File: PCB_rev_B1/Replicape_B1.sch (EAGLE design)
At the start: 233 parts, among them IC1 TMC2100-LA, IC10 74AHC1G126DCK, IC11 74AHC1G126DCK, IC12 TMC2100-LA, IC13 74AHC1G126DCK, IC14 74AHC1G126DCK, IC15 TMC2100-LA, IC16 74AHC1G126DCK, IC17 74AHC1G126DCK, IC2 TMC2100-LA, IC3 74AHC1G126DCK, IC4 74AHC1G126DCK, IC5 TMC2100-LA, IC6 74AHC1G126DCK, IC7 74AHC1G126DCK, IC8 74AHC1G126DCK, IC9 74AHC1G126DCK, P8 F-2X23-, P9 F-2X23-, Q1 AON6758, Q2 AON6758, Q3 AON6758, U1 SN74AHC595PW, U10 RT8268, U11 PCA9685PW, U18 CAT24C256, U19 CD4050BD, U2 SN74AHC595PW, U3 SN74AHC595PW, U4 SN74AHC595PW, U5 SN74AHC595PW, U6 MCP16321, X1 22-05-7038-03, X10 22-05-7038-03, X11 22-05-7028-02, X12 22-05-7048-04, X13 22-05-7038-03, X14 22-05-7048-04, X15 22-05-7048-04, X16 22-05-7048-04, X17 22-05-7048-04, X18 22-05-7048-04, X19 22-05-7038-03, X2 MSTBA4, X20 MSTBA4, X21 MSTBA2, X22 22-05-7038-03, X23 22-05-7038-03, X3 MSTBA2, X4 22-05-7028-02, X5 22-05-7028-02, X6 22-05-7028-02, X7 22-05-7028-02, X8 22-05-7028-02, X9 22-05-7028-02

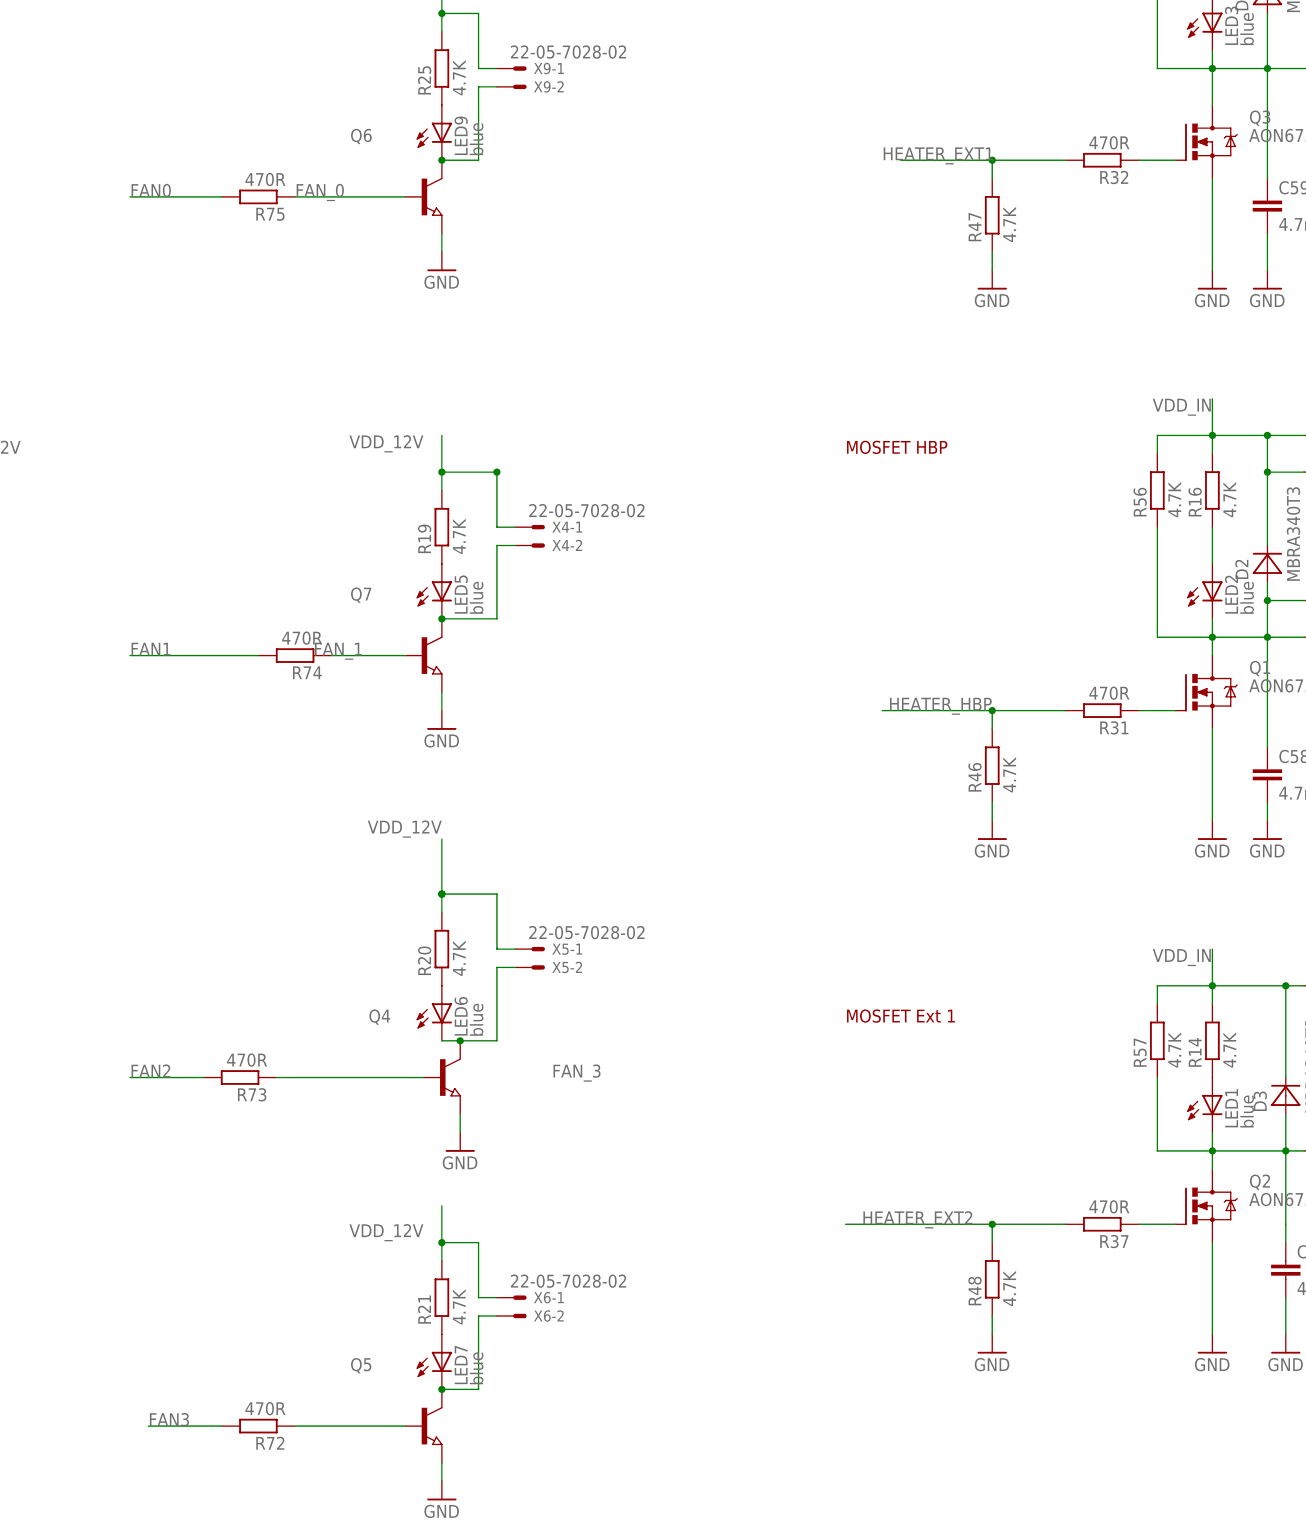
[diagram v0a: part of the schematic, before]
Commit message: Added eagleup
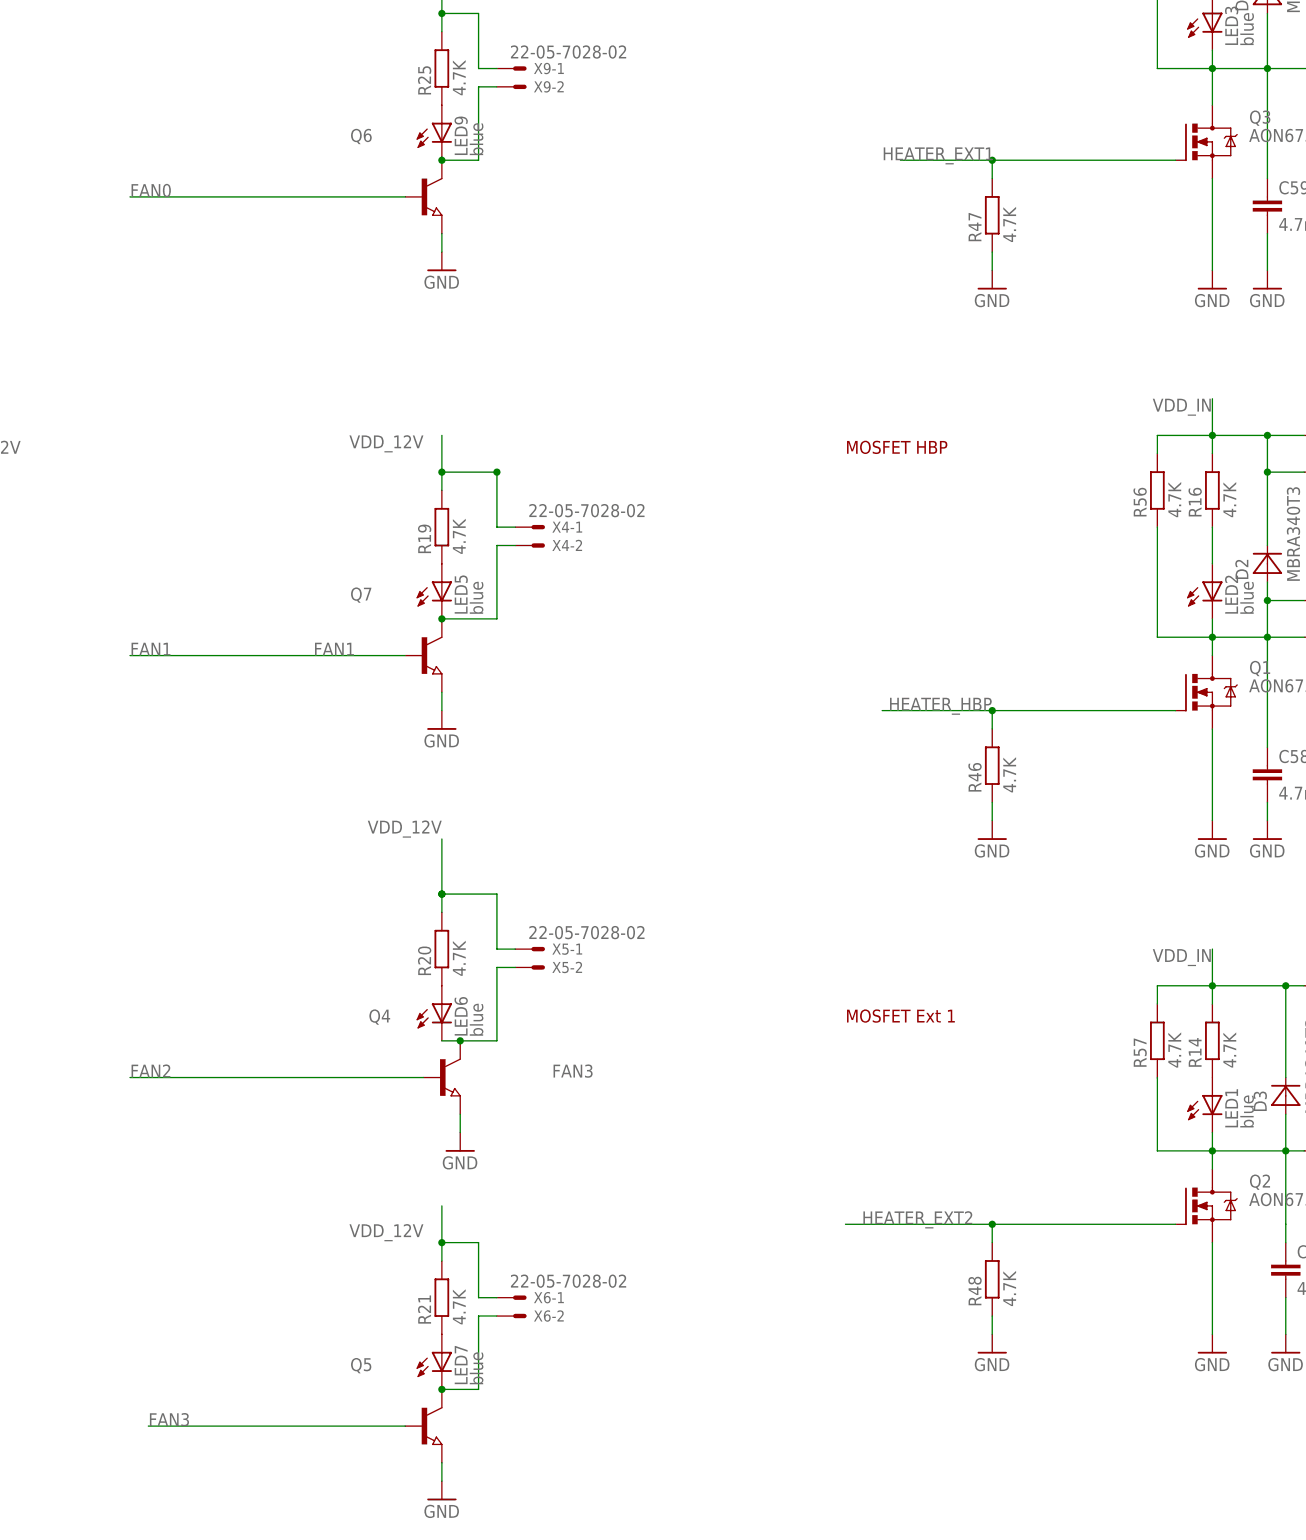
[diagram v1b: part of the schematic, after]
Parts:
- removed R31, R32, R37, R72, R73, R74, R75: 470R, rcl:R-EU_R0402
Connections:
- removed net FAN_0: Q6.B, R75.1
- removed net FAN_1: Q7.B, R74.1
- removed net FAN_2: Q4.B, R73.1
- removed net FAN_3: Q5.B, R72.1
- removed net N$133: Q3.G, R32.1
- removed net N$23: Q2.G, R37.1
- removed net N$60: Q1.G, R31.1
- net FAN0: now also Q6.B; no longer R75.2
- net FAN1: now also Q7.B; no longer R74.2
- net FAN2: now also Q4.B; no longer R73.2
- net FAN3: now also Q5.B; no longer R72.2
- net HEATER_EXT1: now also Q3.G; no longer R32.2
- net HEATER_EXT2: now also Q2.G; no longer R37.2
- net HEATER_HBP: now also Q1.G; no longer R31.2
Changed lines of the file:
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@@
 <part name="GND26" library="supply1" deviceset="GND" device=""/>
 <part name="X14" library="con-molex" deviceset="22-?-04" device="05-7048"/>
-<part name="R32" library="rcl" deviceset="R-EU_" device="R0402" value="470R"/>
-<part name="R31" library="rcl" deviceset="R-EU_" device="R0402" value="470R"/>
 <part name="GND69" library="supply1" deviceset="GND" device=""/>
-<part name="R37" library="rcl" deviceset="R-EU_" device="R0402" value="470R"/>
 <part name="D1" library="diode" deviceset="MBRA340T3" device=""/>
 <part name="D2" library="diode" deviceset="MBRA340T3" device=""/>
@@
 <part name="X12" library="con-molex" deviceset="22-?-04" device="05-7048"/>
 <part name="X23" library="con-molex" deviceset="22-?-03" device="05-7038"/>
-<part name="R72" library="rcl" deviceset="R-EU_" device="R0402" value="470R"/>
-<part name="R73" library="rcl" deviceset="R-EU_" device="R0402" value="470R"/>
-<part name="R74" library="rcl" deviceset="R-EU_" device="R0402" value="470R"/>
-<part name="R75" library="rcl" deviceset="R-EU_" device="R0402" value="470R"/>
 <part name="IC1" library="we-chip" deviceset="TMC2100" device="-LA"/>
 <part name="C2" library="rcl" deviceset="C-EU" device="C0402" value="0.1uF"/>
@@
 <instance part="X21" gate="-1" x="355.6" y="93.98" rot="R180"/>
 <instance part="X21" gate="-2" x="355.6" y="71.12" rot="R180"/>
-<instance part="R32" gate="G$1" x="322.58" y="208.28" rot="R180"/>
-<instance part="R31" gate="G$1" x="322.58" y="132.08" rot="R180"/>
 <instance part="GND69" gate="1" x="337.82" y="43.18"/>
-<instance part="R37" gate="G$1" x="322.58" y="60.96" rot="R180"/>
 <instance part="D1" gate="G$1" x="345.44" y="231.14" rot="R90"/>
 <instance part="D2" gate="G$1" x="345.44" y="152.4" rot="R90"/>
@@
 <instance part="X23" gate="-2" x="444.5" y="195.58" rot="MR0"/>
 <instance part="X23" gate="-3" x="444.5" y="190.5" rot="MR0"/>
-<instance part="R72" gate="G$1" x="205.74" y="33.02" rot="R180"/>
-<instance part="R73" gate="G$1" x="203.2" y="81.28" rot="R180"/>
-<instance part="R74" gate="G$1" x="210.82" y="139.7" rot="R180"/>
-<instance part="R75" gate="G$1" x="205.74" y="203.2" rot="R180"/>
 <instance part="IC1" gate="IC" x="223.52" y="749.3"/>
 <instance part="C2" gate="G$1" x="144.78" y="777.24" rot="MR0"/>
@@
 </segment>
 </net>
-<net name="FAN_1" class="0">
-<segment>
-<pinref part="Q7" gate="G$1" pin="B"/>
-<wire x1="226.06" y1="139.7" x2="215.9" y2="139.7" width="0.1524" layer="91"/>
-<label x="213.36" y="139.7" size="1.778" layer="95"/>
-<pinref part="R74" gate="G$1" pin="1"/>
-</segment>
-</net>
-<net name="FAN_2" class="0">
-<segment>
-<pinref part="Q4" gate="G$1" pin="B"/>
-<wire x1="228.6" y1="81.28" x2="208.28" y2="81.28" width="0.1524" layer="91"/>
-<pinref part="R73" gate="G$1" pin="1"/>
-</segment>
-</net>
-<net name="FAN_3" class="0">
-<segment>
-<label x="246.38" y="81.28" size="1.778" layer="95"/>
-<pinref part="Q5" gate="G$1" pin="B"/>
-<wire x1="226.06" y1="33.02" x2="210.82" y2="33.02" width="0.1524" layer="91"/>
-<pinref part="R72" gate="G$1" pin="1"/>
-</segment>
-</net>
 <net name="+3V3" class="0">
 <segment>
@@
 <pinref part="R48" gate="G$1" pin="2"/>
 <junction x="307.34" y="60.96"/>
-<pinref part="R37" gate="G$1" pin="2"/>
-<wire x1="307.34" y1="60.96" x2="317.5" y2="60.96" width="0.1524" layer="91"/>
+<pinref part="Q2" gate="Q" pin="G"/>
+<wire x1="307.34" y1="60.96" x2="332.74" y2="60.96" width="0.1524" layer="91"/>
 </segment>
 </net>
@@
 <pinref part="R46" gate="G$1" pin="2"/>
 <junction x="307.34" y="132.08"/>
-<pinref part="R31" gate="G$1" pin="2"/>
-<wire x1="307.34" y1="132.08" x2="317.5" y2="132.08" width="0.1524" layer="91"/>
+<pinref part="Q1" gate="Q" pin="G"/>
+<wire x1="307.34" y1="132.08" x2="332.74" y2="132.08" width="0.1524" layer="91"/>
 </segment>
 </net>
@@
 <label x="292.1" y="208.28" size="1.778" layer="95"/>
 <pinref part="R47" gate="G$1" pin="2"/>
-<pinref part="R32" gate="G$1" pin="2"/>
-<wire x1="317.5" y1="208.28" x2="307.34" y2="208.28" width="0.1524" layer="91"/>
 <junction x="307.34" y="208.28"/>
+<pinref part="Q3" gate="Q" pin="G"/>
+<wire x1="307.34" y1="208.28" x2="332.74" y2="208.28" width="0.1524" layer="91"/>
 </segment>
 </net>
@@
 </segment>
 </net>
-<net name="N$133" class="0">
-<segment>
-<wire x1="332.74" y1="208.28" x2="327.66" y2="208.28" width="0.1524" layer="91"/>
-<pinref part="R32" gate="G$1" pin="1"/>
-<pinref part="Q3" gate="Q" pin="G"/>
-</segment>
-</net>
-<net name="N$60" class="0">
-<segment>
-<wire x1="332.74" y1="132.08" x2="327.66" y2="132.08" width="0.1524" layer="91"/>
-<pinref part="R31" gate="G$1" pin="1"/>
-<pinref part="Q1" gate="Q" pin="G"/>
-</segment>
-</net>
 <net name="N$242" class="0">
 <segment>
@@
 </segment>
 </net>
-<net name="N$23" class="0">
-<segment>
-<wire x1="332.74" y1="60.96" x2="327.66" y2="60.96" width="0.1524" layer="91"/>
-<pinref part="R37" gate="G$1" pin="1"/>
-<pinref part="Q2" gate="Q" pin="G"/>
-</segment>
-</net>
 <net name="SPI1_SCLK" class="0">
 <segment>
@@
 </segment>
 </net>
-<net name="FAN_0" class="0">
-<segment>
-<label x="210.82" y="203.2" size="1.778" layer="95"/>
-<wire x1="226.06" y1="203.2" x2="210.82" y2="203.2" width="0.1524" layer="91"/>
-<pinref part="Q6" gate="G$1" pin="B"/>
-<pinref part="R75" gate="G$1" pin="1"/>
-</segment>
-</net>
 <net name="FAN0" class="0">
 <segment>
-<pinref part="R75" gate="G$1" pin="2"/>
-<wire x1="200.66" y1="203.2" x2="187.96" y2="203.2" width="0.1524" layer="91"/>
+<wire x1="226.06" y1="203.2" x2="187.96" y2="203.2" width="0.1524" layer="91"/>
 <label x="187.96" y="203.2" size="1.778" layer="95"/>
+<pinref part="Q6" gate="G$1" pin="B"/>
 </segment>
 <segment>
@@
 <net name="FAN1" class="0">
 <segment>
-<pinref part="R74" gate="G$1" pin="2"/>
-<wire x1="205.74" y1="139.7" x2="187.96" y2="139.7" width="0.1524" layer="91"/>
+<wire x1="226.06" y1="139.7" x2="187.96" y2="139.7" width="0.1524" layer="91"/>
 <label x="187.96" y="139.7" size="1.778" layer="95"/>
+<pinref part="Q7" gate="G$1" pin="B"/>
+<label x="213.36" y="139.7" size="1.778" layer="95"/>
 </segment>
 <segment>
@@
 <net name="FAN2" class="0">
 <segment>
-<pinref part="R73" gate="G$1" pin="2"/>
-<wire x1="198.12" y1="81.28" x2="187.96" y2="81.28" width="0.1524" layer="91"/>
 <label x="187.96" y="81.28" size="1.778" layer="95"/>
+<pinref part="Q4" gate="G$1" pin="B"/>
+<wire x1="187.96" y1="81.28" x2="228.6" y2="81.28" width="0.1524" layer="91"/>
 </segment>
 <segment>
@@
 <net name="FAN3" class="0">
 <segment>
-<pinref part="R72" gate="G$1" pin="2"/>
-<wire x1="200.66" y1="33.02" x2="190.5" y2="33.02" width="0.1524" layer="91"/>
 <label x="190.5" y="33.02" size="1.778" layer="95"/>
+<label x="246.38" y="81.28" size="1.778" layer="95"/>
+<pinref part="Q5" gate="G$1" pin="B"/>
+<wire x1="190.5" y1="33.02" x2="226.06" y2="33.02" width="0.1524" layer="91"/>
 </segment>
 <segment>
